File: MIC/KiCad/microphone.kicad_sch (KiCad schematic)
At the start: 17 parts, among them J1 Conn_01x06_Pin, U1 LMV321

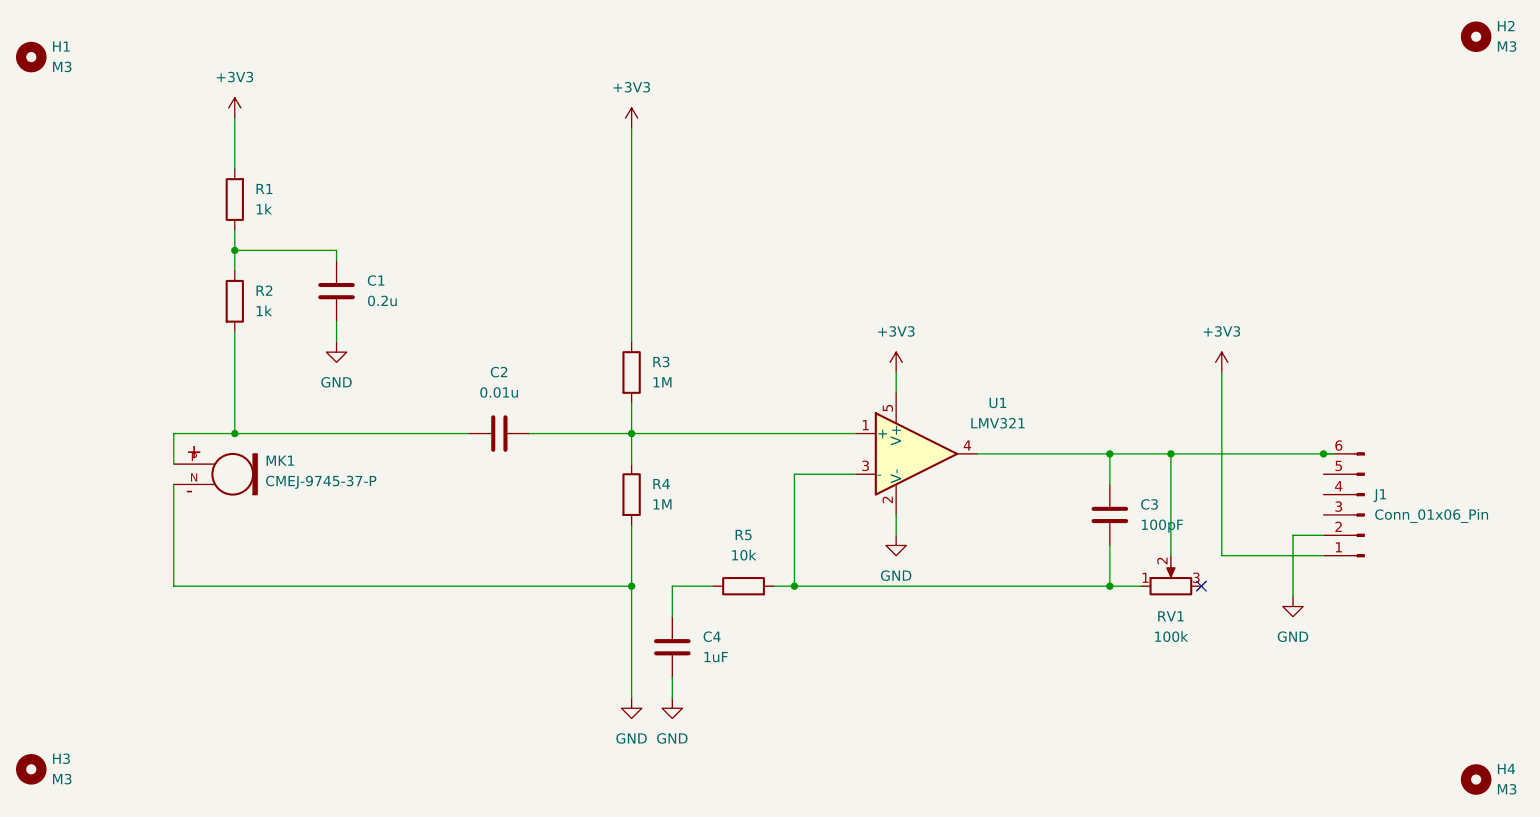
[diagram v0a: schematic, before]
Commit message: Deployed d972a79 with MkDocs version: 1.6.0
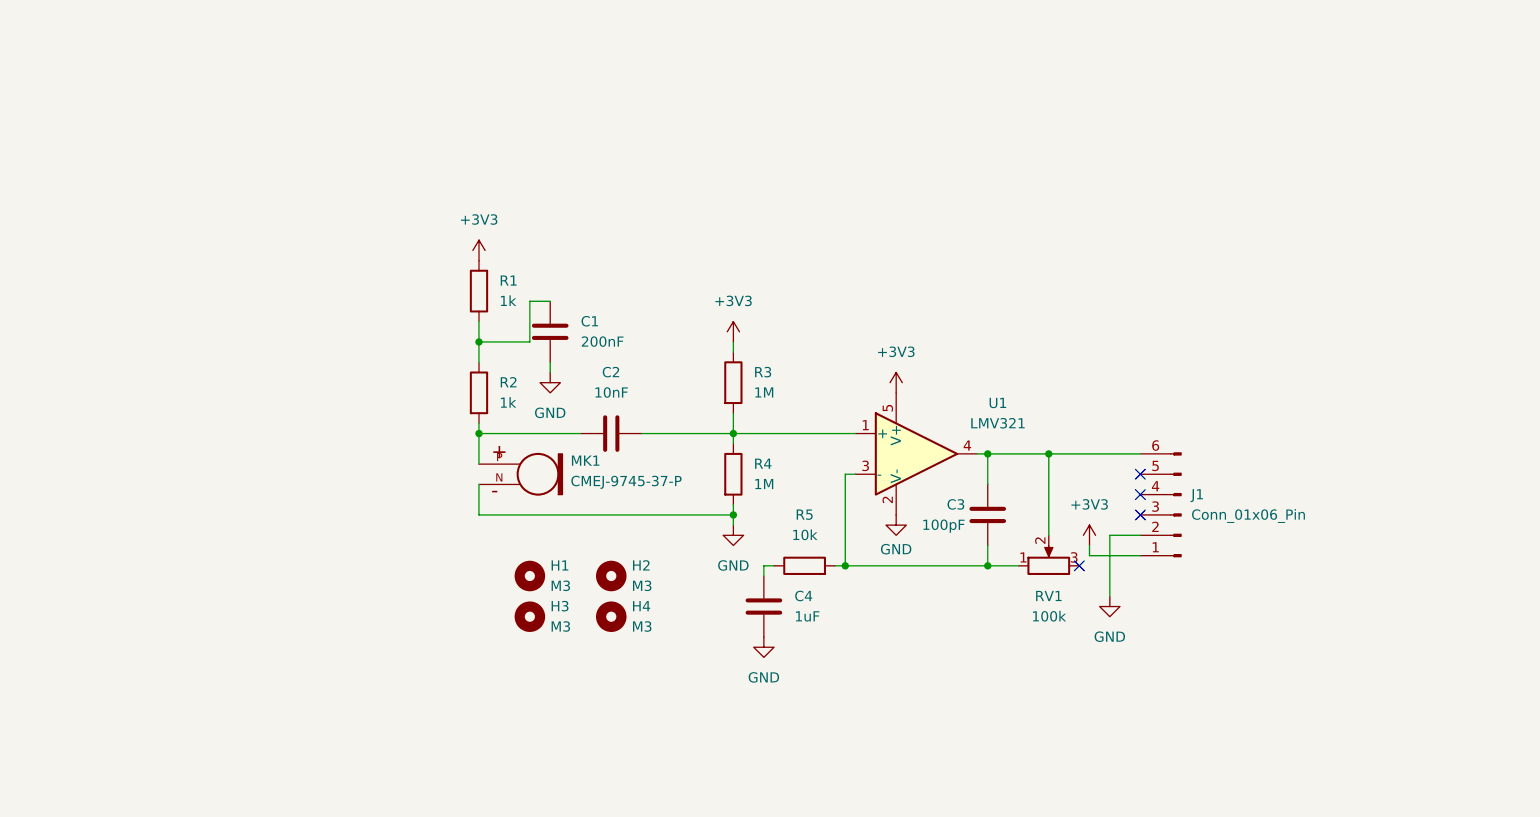
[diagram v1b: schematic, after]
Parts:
- C1: value 0.2u -> 200nF
- C2: value 0.01u -> 10nF
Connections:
- no-connect marks 1 -> 4
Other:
- moved on the sheet: C1, C2, C3, C4, H1, H2, H3, H4, J1, MK1, R1, R2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
